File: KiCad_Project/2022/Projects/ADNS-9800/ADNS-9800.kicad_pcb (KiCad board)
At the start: 2 copper layers, 42 x 27.3 mm, 15 parts, among them J1 Conn_01x04, Q1 IRLML6402, U1 SeeeduinoXIAO

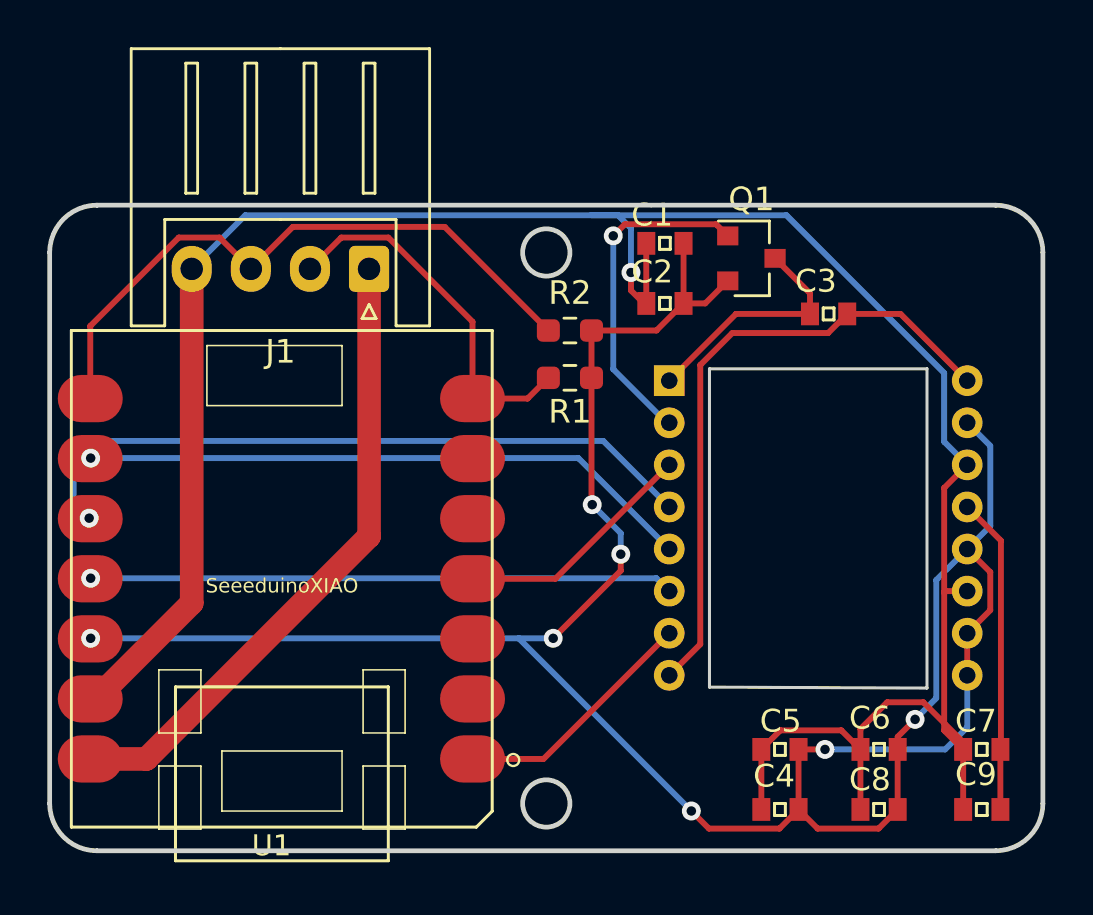
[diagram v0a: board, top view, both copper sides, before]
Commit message: マウス基板の改良
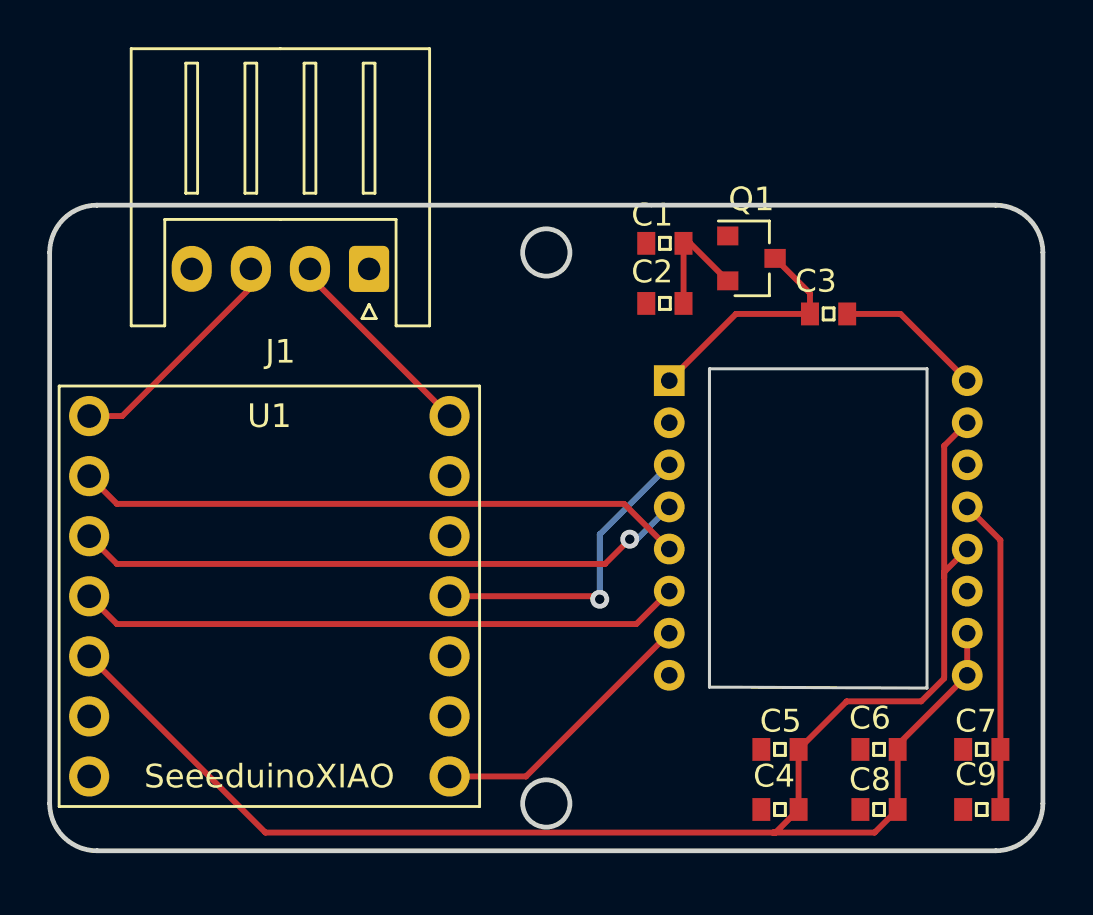
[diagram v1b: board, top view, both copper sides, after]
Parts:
- removed R1, R2: R, Resistor_SMD:R_0603_1608Metric_Pad0.98x0.95mm_HandSolder
- U1: footprint Library:Seeeduino XIAO-MOUDLE14P-2.54-21X17.8MM -> Library:seeeduinoXIAO
- moved U1 14.7 mm to (150.8, 83.0), turned to 0 degrees
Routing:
- net GND: track 100.8 -> 0.00 mm, vias 1 -> 0
- net +5V: track 27.0 -> 0.00 mm
- net +3V3: track 100.6 -> 75.7 mm, vias 7 -> 0
- net Net-(C3-Pad1): track 27.0 -> 6.24 mm
- net RX: track 27.1 -> 9.87 mm
- net /LSR_NEN: track 14.2 -> 0.00 mm, vias 1 -> 0
- net TX: track 15.7 -> 8.67 mm
- net /MISO: track 29.7 -> 26.0 mm
- net /SS: track 10.3 -> 13.3 mm, vias 0 -> 1
- net /MOTION: track 10.5 -> 11.8 mm
- net /MOSI: track 24.7 -> 25.6 mm, vias 1 -> 0
- net /SCLK: track 26.1 -> 25.8 mm, vias 1 -> 0
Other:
- net class Default removed
